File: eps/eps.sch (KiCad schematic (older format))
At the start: 0 parts

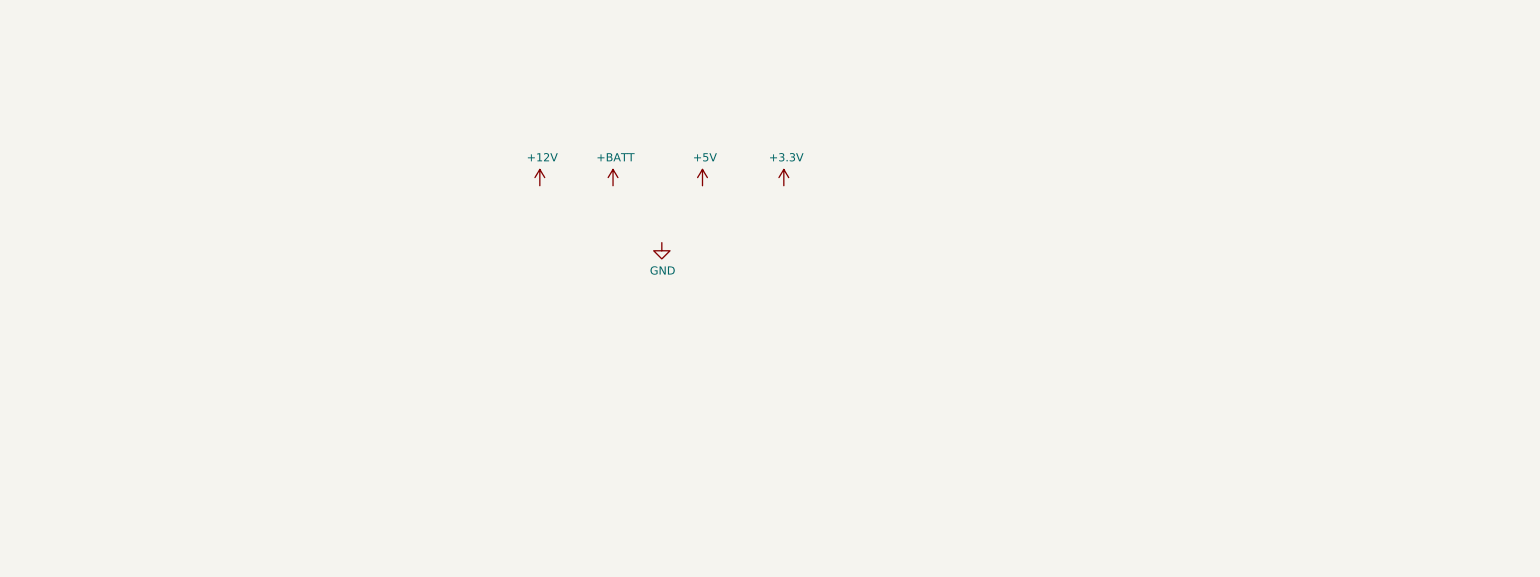
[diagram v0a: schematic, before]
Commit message: fourteen mosfets
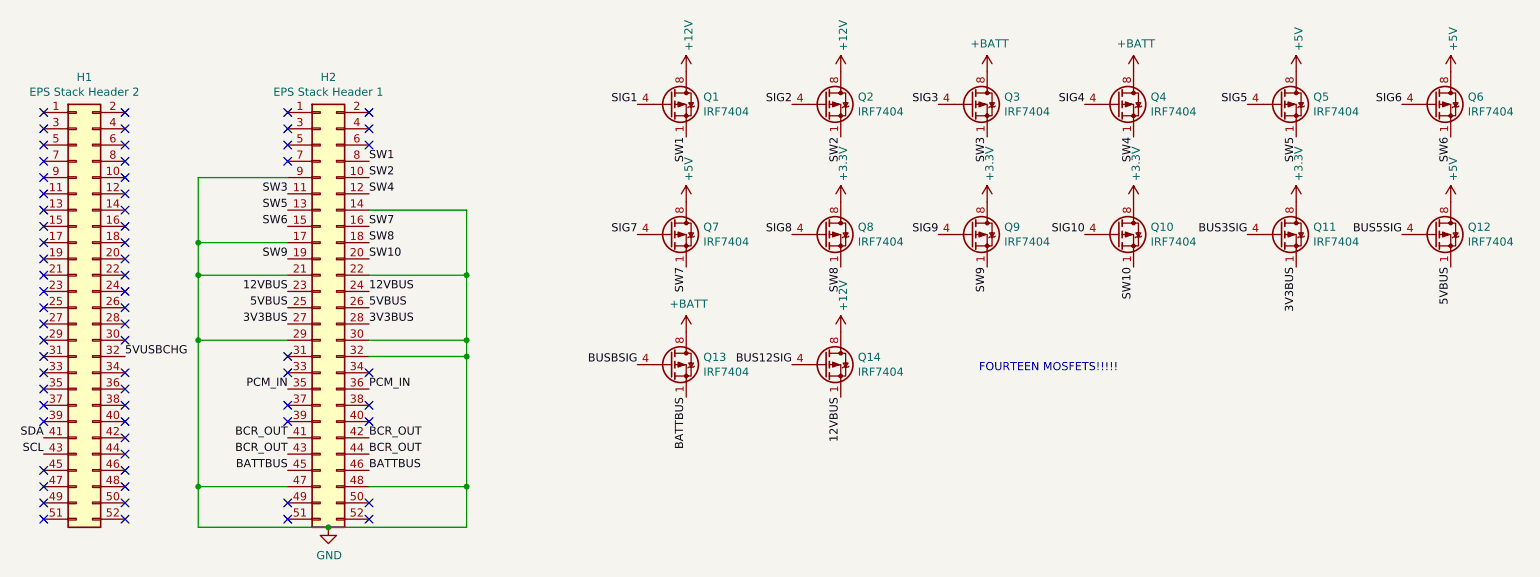
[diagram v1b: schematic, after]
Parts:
- added H1: EPS Stack Header 2, symbol Connector_Generic:Conn_02x26_Odd_Even
- added H2: EPS Stack Header 1, symbol Connector_Generic:Conn_02x26_Odd_Even
- added Q1, Q10, Q11, Q12, Q13, Q14, Q2, Q3, Q4, Q5, Q6, Q7, Q8, Q9: IRF7404, Package_SO:SOIC-8_3.9x4.9mm_P1.27mm, symbol Transistor_FET:IRF7404
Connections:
- net +12V: now also Q1.5 (D), Q1.6 (D), Q1.7 (D), Q1.8 (D), Q14.5 (D), Q14.6 (D), Q14.7 (D), Q14.8 (D), Q2.5 (D), Q2.6 (D), Q2.7 (D), Q2.8 (D)
- net +3V3: now also Q10.5 (D), Q10.6 (D), Q10.7 (D), Q10.8 (D), Q11.5 (D), Q11.6 (D), Q11.7 (D), Q11.8 (D), Q8.5 (D), Q8.6 (D), Q8.7 (D), Q8.8 (D), Q9.5 (D), Q9.6 (D), Q9.7 (D), Q9.8 (D)
- net +5V: now also Q12.5 (D), Q12.6 (D), Q12.7 (D), Q12.8 (D), Q5.5 (D), Q5.6 (D), Q5.7 (D), Q5.8 (D), Q6.5 (D), Q6.6 (D), Q6.7 (D), Q6.8 (D), Q7.5 (D), Q7.6 (D), Q7.7 (D), Q7.8 (D)
- net +BATT: now also Q13.5 (D), Q13.6 (D), Q13.7 (D), Q13.8 (D), Q3.5 (D), Q3.6 (D), Q3.7 (D), Q3.8 (D), Q4.5 (D), Q4.6 (D), Q4.7 (D), Q4.8 (D)
- net GND: now also H2.14 (Pin_14), H2.17 (Pin_17), H2.21 (Pin_21), H2.22 (Pin_22), H2.29 (Pin_29), H2.30 (Pin_30), H2.32 (Pin_32), H2.47 (Pin_47), H2.48 (Pin_48), H2.9 (Pin_9)
- new net 12VBUS: H2.23 (Pin_23), H2.24 (Pin_24), Q14.1 (S), Q14.2 (S), Q14.3 (S)
- new net 3V3BUS: H2.27 (Pin_27), H2.28 (Pin_28), Q11.1 (S), Q11.2 (S), Q11.3 (S)
- new net 5VBUS: H2.25 (Pin_25), H2.26 (Pin_26), Q12.1 (S), Q12.2 (S), Q12.3 (S)
- new net 5VUSBCHG: H1.32 (Pin_32)
- new net BATTBUS: H2.45 (Pin_45), H2.46 (Pin_46), Q13.1 (S), Q13.2 (S), Q13.3 (S)
- new net BCR_OUT: H2.41 (Pin_41), H2.42 (Pin_42), H2.43 (Pin_43), H2.44 (Pin_44)
- new net BUS12SIG: Q14.4 (G)
- new net BUS3SIG: Q11.4 (G)
- new net BUS5SIG: Q12.4 (G)
- new net BUSBSIG: Q13.4 (G)
- new net PCM_IN: H2.35 (Pin_35), H2.36 (Pin_36)
- new net SCL: H1.43 (Pin_43)
- new net SDA: H1.41 (Pin_41)
- new net SIG1: Q1.4 (G)
- new net SIG10: Q10.4 (G)
- new net SIG2: Q2.4 (G)
- new net SIG3: Q3.4 (G)
- new net SIG4: Q4.4 (G)
- new net SIG5: Q5.4 (G)
- new net SIG6: Q6.4 (G)
- new net SIG7: Q7.4 (G)
- new net SIG8: Q8.4 (G)
- new net SIG9: Q9.4 (G)
- new net SW1: H2.8 (Pin_8), Q1.1 (S), Q1.2 (S), Q1.3 (S)
- new net SW10: H2.20 (Pin_20), Q10.1 (S), Q10.2 (S), Q10.3 (S)
- new net SW2: H2.10 (Pin_10), Q2.1 (S), Q2.2 (S), Q2.3 (S)
- new net SW3: H2.11 (Pin_11), Q3.1 (S), Q3.2 (S), Q3.3 (S)
- new net SW4: H2.12 (Pin_12), Q4.1 (S), Q4.2 (S), Q4.3 (S)
- new net SW5: H2.13 (Pin_13), Q5.1 (S), Q5.2 (S), Q5.3 (S)
- new net SW6: H2.15 (Pin_15), Q6.1 (S), Q6.2 (S), Q6.3 (S)
- new net SW7: H2.16 (Pin_16), Q7.1 (S), Q7.2 (S), Q7.3 (S)
- new net SW8: H2.18 (Pin_18), Q8.1 (S), Q8.2 (S), Q8.3 (S)
- new net SW9: H2.19 (Pin_19), Q9.1 (S), Q9.2 (S), Q9.3 (S)
- no-connect marks 0 -> 67
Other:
- note added: "FOURTEEN MOSFETS!!!!!"
